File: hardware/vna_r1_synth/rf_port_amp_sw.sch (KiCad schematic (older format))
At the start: 16 parts

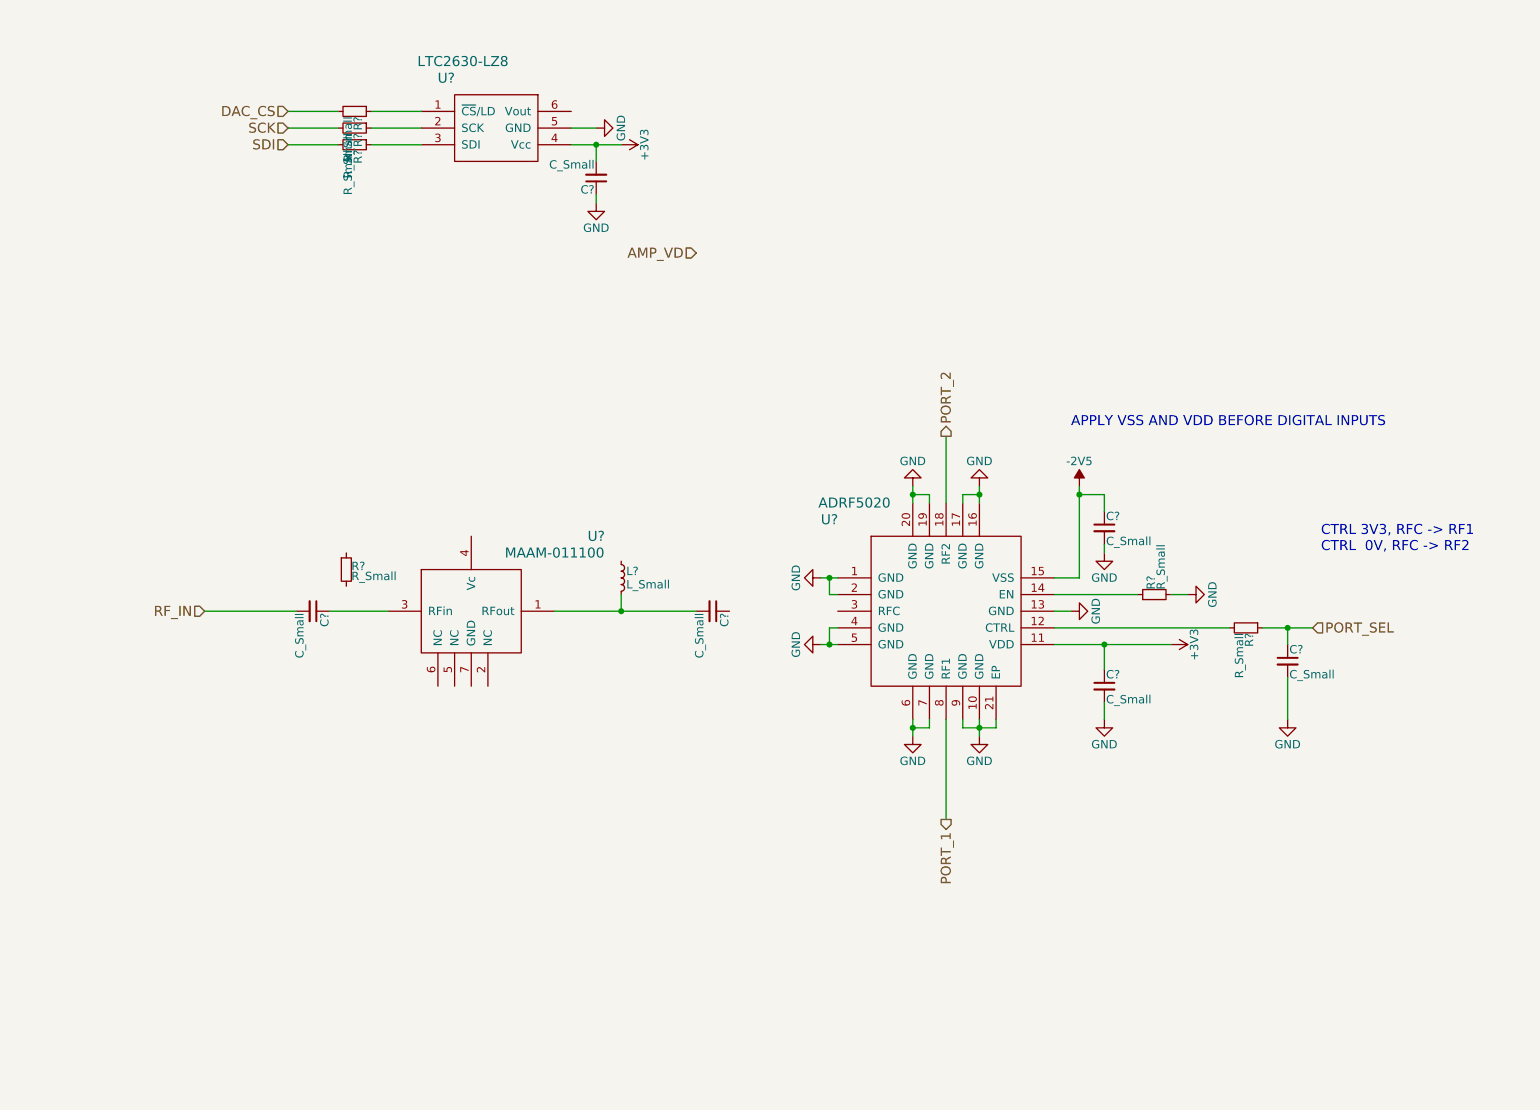
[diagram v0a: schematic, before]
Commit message: work on vna r1 synth schematic
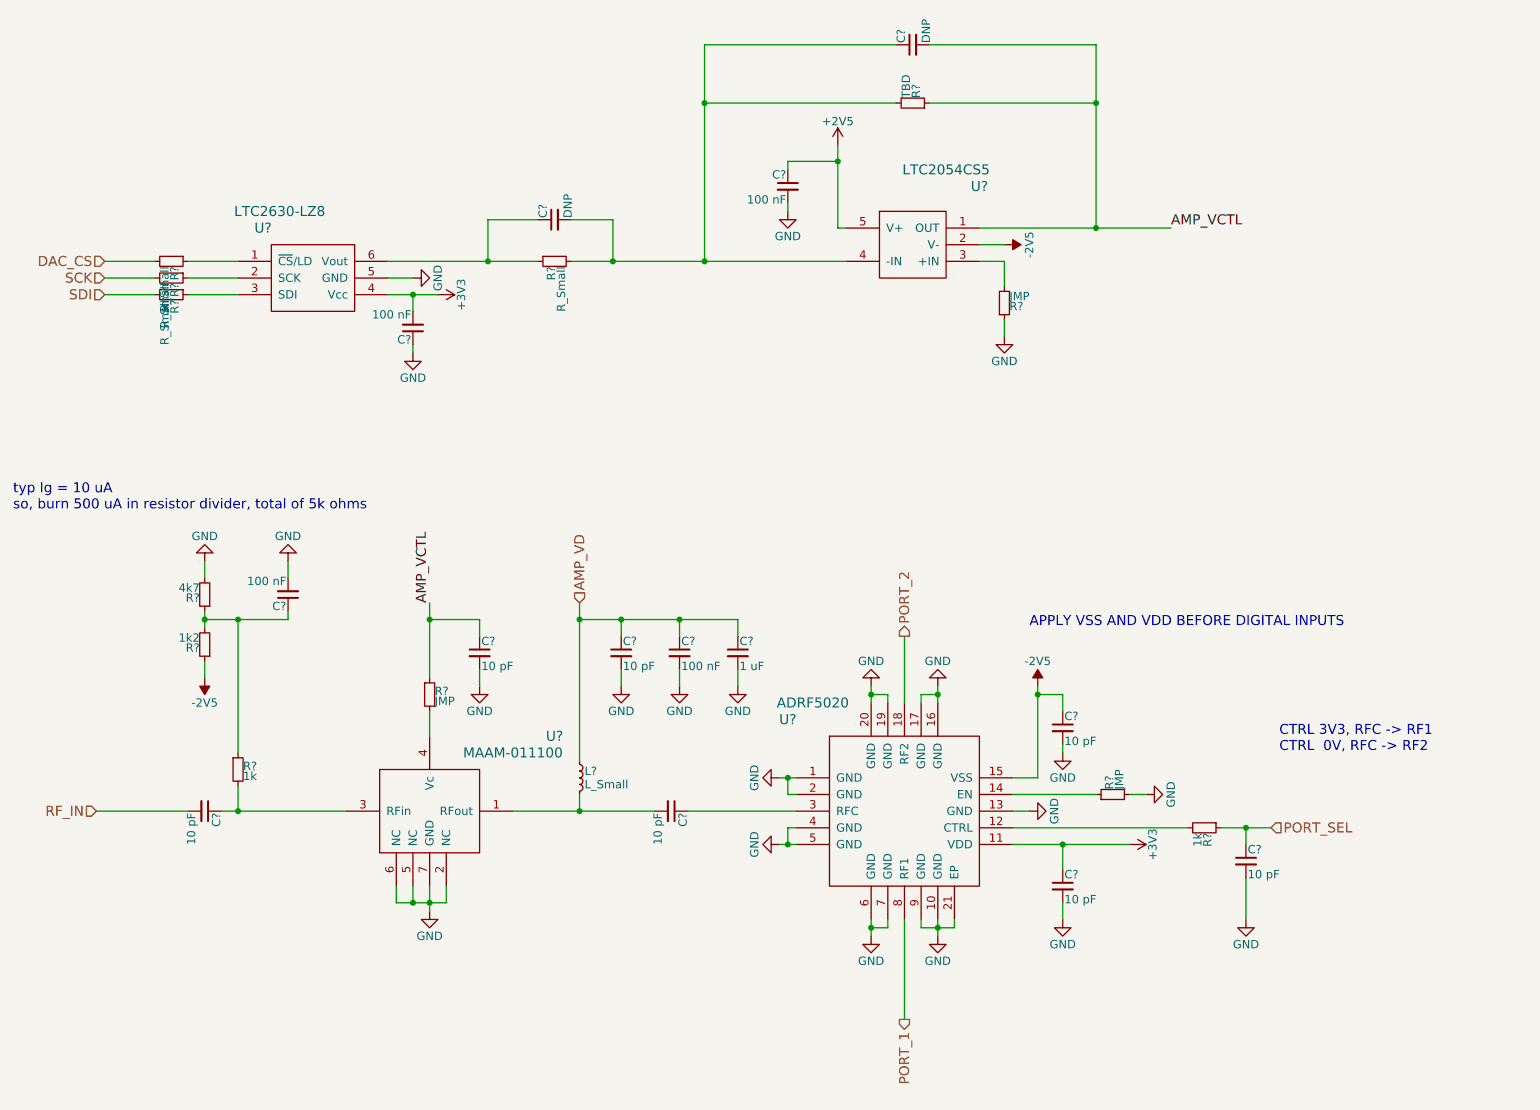
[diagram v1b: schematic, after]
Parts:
- added C? (x3): 100 nF, symbol C_Small
- added C? (x2): 10 pF, symbol C_Small
- added C?: 1 uF, symbol C_Small
- added C? (x2): DNP, symbol C_Small
- added R?: 4k7, symbol R_Small
- added R?: 1k2, symbol R_Small
- added R? (x2): JMP, symbol R_Small
- added R?: R_Small, symbol R_Small
- added R?: TBD, symbol R_Small
- added U?: LTC2054CS5, symbol LTC2054CS5
- C? (x5): value C_Small -> 10 pF
- C?: value C_Small -> 100 nF
- R? (x2): value R_Small -> 1k
- R?: value R_Small -> JMP
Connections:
- net -2V5: now also R?.1, U?.2 (V-)
- net AMP_VD: now also L?.1, C?.1, C?.1, C?.1
- net GND: now also U?.2 (NC), U?.5 (NC), U?.6 (NC), U?.7 (GND), C?.2, C?.2, C?.2, C?.2, C?.2, C?.2, R?.1, R?.2
- net at U?.3 (RFC): now also C?.1
- net at C?.1, U?.3 (RFin): now also R?.2
- net at U?.4 (Vc): now also R?.2
- net at R?.1: now also C?.1, R?.1, R?.2
- net at U?.6 (Vout): now also C?.1, R?.1
- new net: R?.2, U?.3 (+IN)
- new net: C?.1, C?.2, R?.2, R?.2, U?.4 (-IN)
- new net +2V5: C?.1, U?.5 (V+)
- new net AMP_VCTL: C?.1, C?.2, R?.1, R?.1, U?.1 (OUT)
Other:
- note added: "typ Ig = 10 uA\nso, burn 500 uA in resistor divider, total of 5k ohms"
- moved on the sheet: C?, L?, R?, U?
